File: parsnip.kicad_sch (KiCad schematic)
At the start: 76 parts, among them J1 SPI BUS, J14 GPIO_Expander, J2 I2C3, J3 I2C1, J4 I2C2, J5 e-Ink Display Connector, J6 UART0, SW1 ESP_RESET, SW2 BOOT, U1 ESP32-S3-WROOM-1, U17 TCAL9539RTWR_C22445413, U2 QMC6309, Y1 32.768KHz

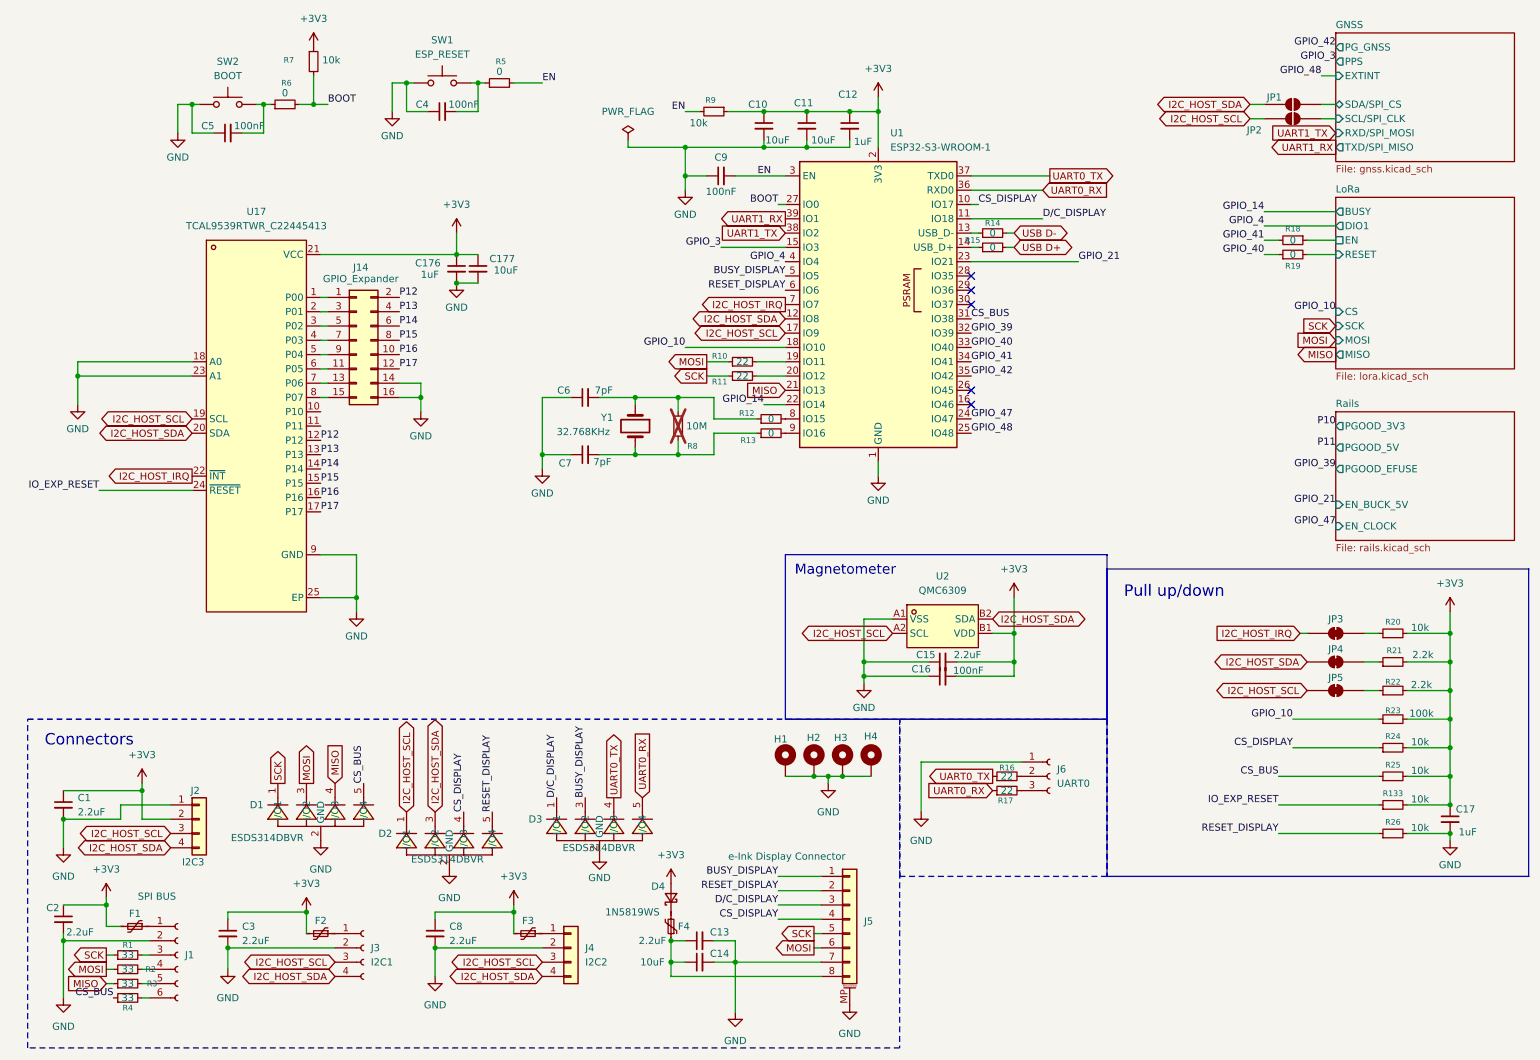
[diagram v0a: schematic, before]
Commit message: organize repo and schematic
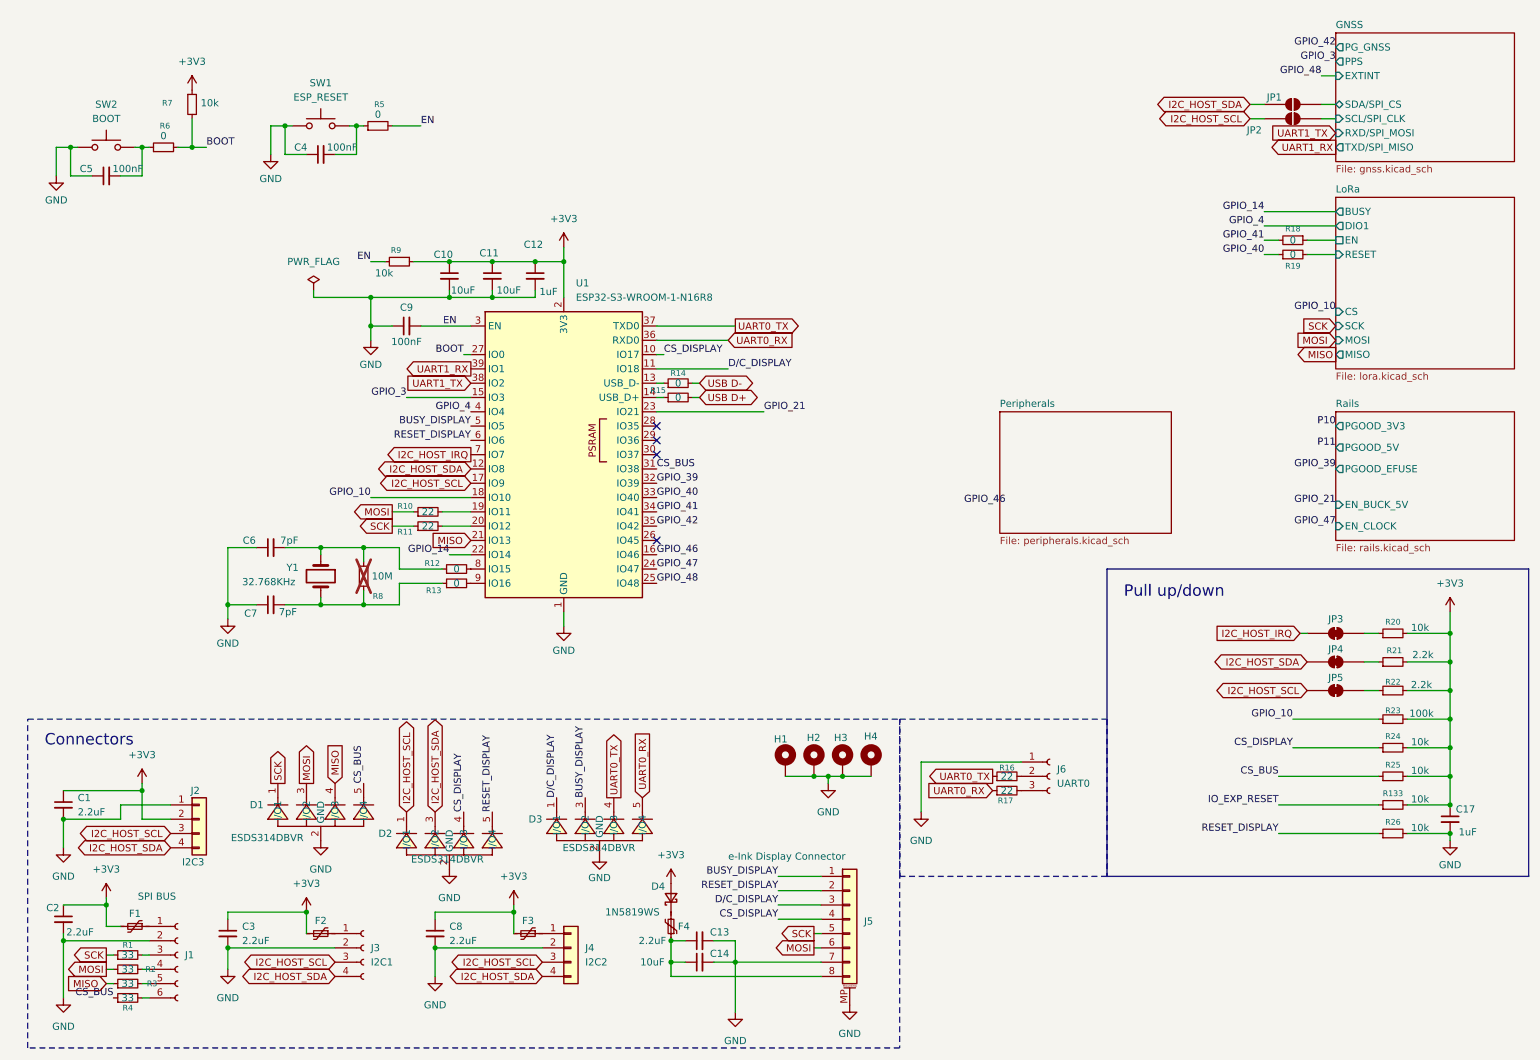
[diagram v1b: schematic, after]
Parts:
- removed C15: 2.2uF, Capacitor_SMD:C_0402_1005Metric, symbol Device:C_Small
- removed C16: 100nF, Capacitor_SMD:C_0402_1005Metric, symbol Device:C_Small
- removed C176: 1uF, Capacitor_SMD:C_0402_1005Metric, symbol Device:C_Small
- removed C177: 10uF, Capacitor_SMD:C_0603_1608Metric, symbol Device:C_Small
- removed J14: GPIO_Expander, Connector_PinSocket_2.54mm:PinSocket_2x08_P2.54mm_Horizontal, symbol Connector_Generic:Conn_02x08_Odd_Even
- removed U17: TCAL9539RTWR_C22445413, easyeda2kicad:TQFN-24_L4.0-W4.0-P0.50-BL-EP2.3, symbol easyeda2kicad:TCAL9539RTWR_C22445413
- removed U2: QMC6309, easyeda2kicad:X1-WLB0808-4_L0.8-W0.8-P0.40-TL, symbol easyeda2kicad:QMC6309
- U1: value ESP32-S3-WROOM-1 -> ESP32-S3-WROOM-1-N16R8
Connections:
- net GPIO_46: now reaches U1.16 (IO46)
- no-connect marks 5 -> 4
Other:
- added sheet Peripherals (peripherals.kicad_sch)
- note removed: "Magnetometer"
- moved on the sheet: C10, C11, C12, C4, C5, C6, C7, C9, R10, R11, R12, R13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
